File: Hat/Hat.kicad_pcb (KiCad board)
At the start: 2 copper layers, 185.8 x 128.5 mm, 102 parts, among them J1 Conn_01x01_Pin, J2 Conn_01x12_Pin, J3 Conn_01x12_Pin, J4 Conn_01x06_Pin, J5 Conn_01x01_Pin, Q1 BC547, Q10 BC547, Q11 BC547, Q12 BC557, Q13 BC547, Q14 BC547, Q15 BC547, Q2 BC547, Q3 BC547, Q4 BC557, Q5 BC557, Q6 BC547, Q7 BC547, Q8 BC547, Q9 BC547, SW1 SW_Push, SW2 SW_SPDT, U1 TL074, U2 Aux_flush, U3 Aux_flush, U4 Aux_flush, U5 4066, U6 Aux_flush, U7 Aux_flush

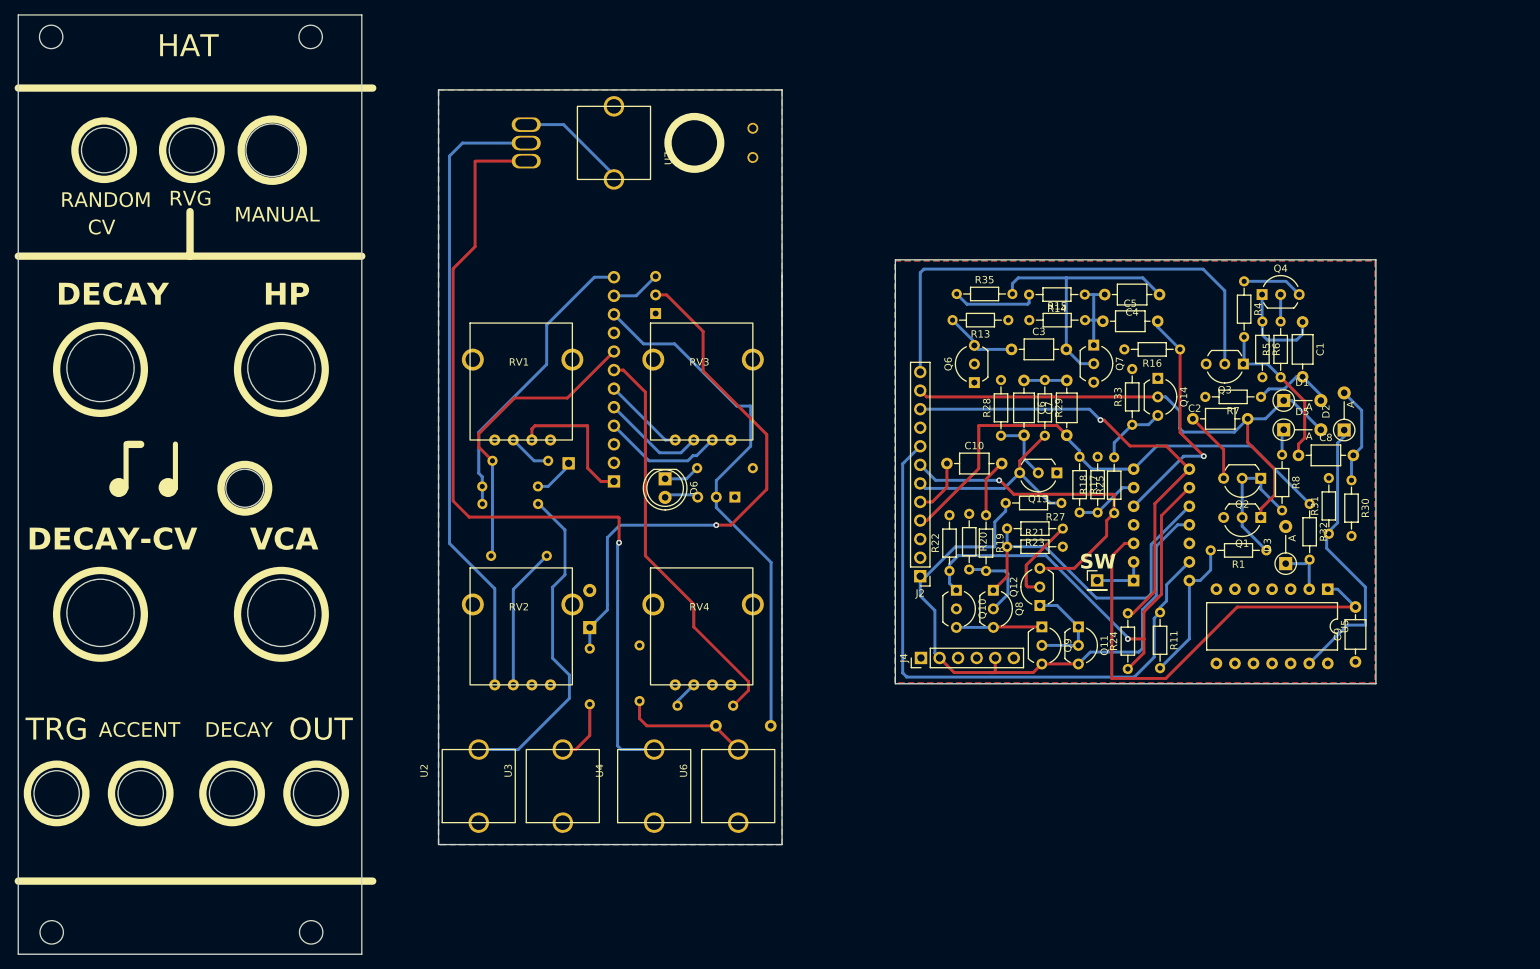
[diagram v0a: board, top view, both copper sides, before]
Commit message: Add files via upload
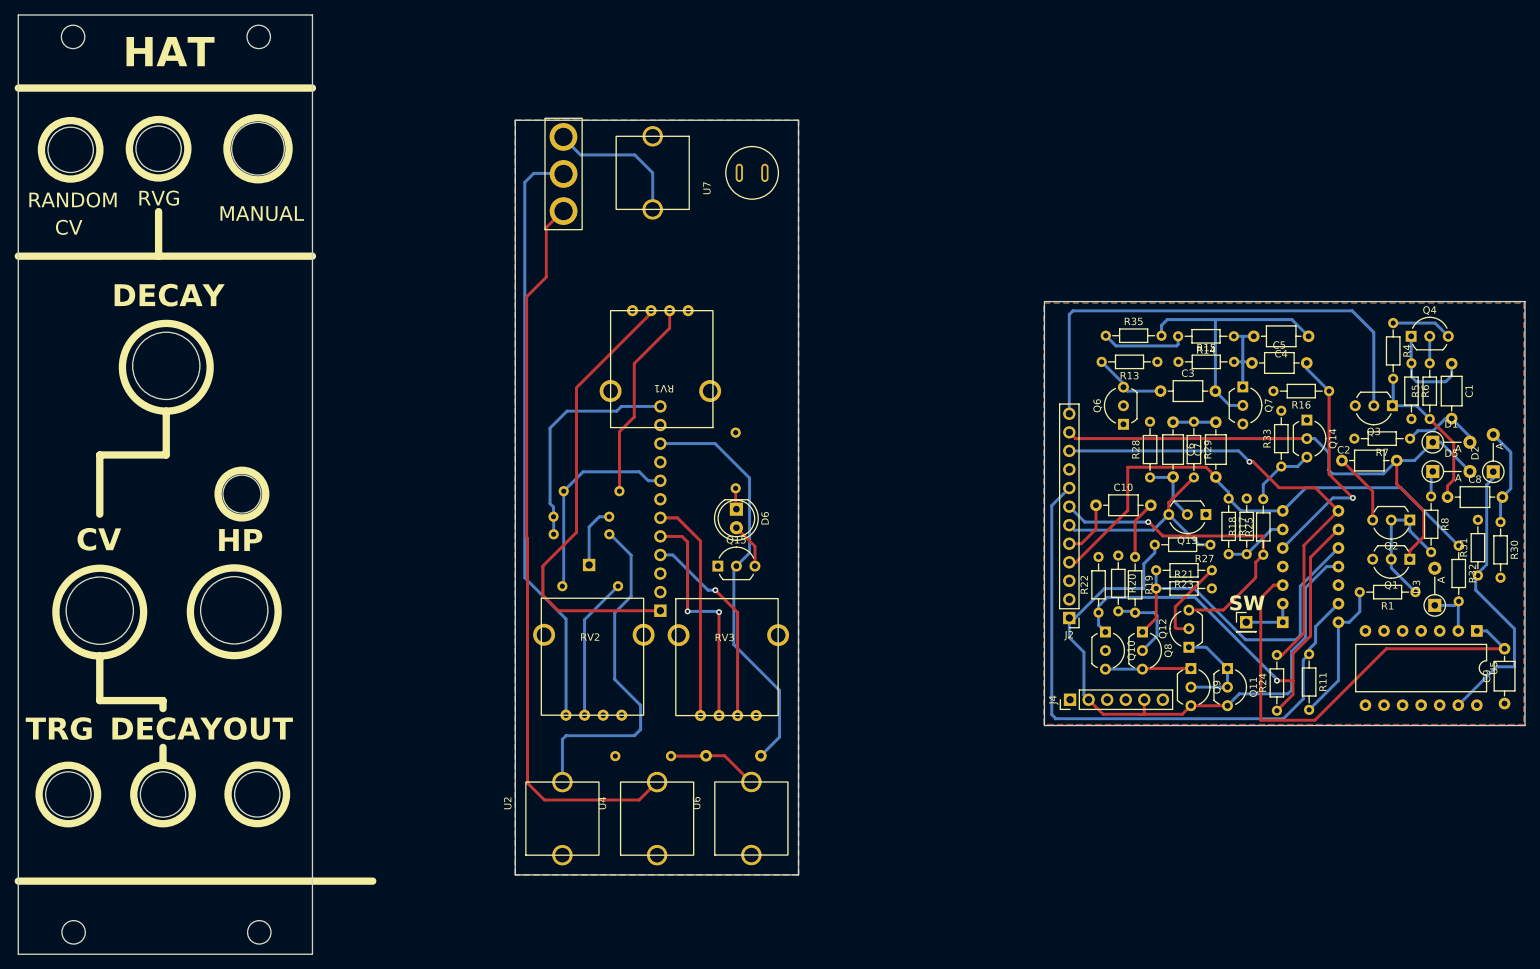
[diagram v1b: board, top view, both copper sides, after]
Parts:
- removed D4: D, Diode_THT:D_A-405_P5.08mm_Vertical_AnodeUp
- removed Q5: BC557, Package_TO_SOT_THT:TO-92_Inline_Wide
- removed R26: 100k, Resistor_THT:R_Axial_DIN0204_L3.6mm_D1.6mm_P7.62mm_Horizontal
- removed R9: 1k, Resistor_THT:R_Axial_DIN0204_L3.6mm_D1.6mm_P7.62mm_Horizontal
- removed the REF** at (59.2, 127.0)
- removed the REF** at (78.5, 68.8)
- removed RV4: R_Potentiometer, Library:AlpsPot
- removed U3: Aux_flush, Library:3mm5 Mono Aux
- Q15: moved to F.Cu
- SW1: footprint Library:Push_Flush -> Library:PushButton
- SW2: footprint Library:SPDT Mini -> Library:Switch
- moved RV3 37.9 mm to (135.8, 116.3)
- moved RV1 31.8 mm to (134.2, 61.0), turned to 180 degrees
- moved C5 21.2 mm to (211.3, 68.1)
- moved D2 21.2 mm to (244.3, 83.0)
- moved D3 21.2 mm to (236.3, 101.3)
- moved J4 21.2 mm to (186.4, 114.2)
- moved Q10 21.2 mm to (191.2, 104.9)
- moved Q11 21.2 mm to (207.9, 109.9)
- moved Q14 21.2 mm to (218.8, 75.9)
- moved Q8 21.2 mm to (196.3, 104.9)
- moved Q9 21.2 mm to (202.9, 109.9)
- moved R11 21.2 mm to (219.1, 108.0)
- moved R19 21.2 mm to (195.3, 94.7)
- moved R23 21.2 mm to (205.8, 96.5)
- moved R27 21.2 mm to (205.6, 93.0)
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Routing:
- net Net-(D4-K): track 74.5 -> 0.00 mm, vias 1 -> 0
- net OFFSET: track 100.4 -> 45.2 mm
- net -12V: track 103.3 -> 145.9 mm
- net Net-(R10-Pad1): track 5.95 -> 27.5 mm
- net NOISE_HP: track 40.0 -> 59.4 mm
- net NOISE_TONED: track 22.0 -> 39.8 mm, vias 0 -> 2
- net OUT: track 136.9 -> 120.6 mm
- net Net-(SW2-A): track 114.8 -> 100.9 mm, vias 1 -> 0
- net VGND: track 123.5 -> 110.7 mm
- net NOISE: track 86.5 -> 97.8 mm, vias 0 -> 1
- net IN: track 107.2 -> 97.8 mm
- net Net-(R9-Pad2): track 8.74 -> 0.00 mm
- net CAP: track 84.6 -> 77.8 mm
- net Net-(C11-Pad2): track 17.8 -> 12.5 mm
- net Net-(SW2-B): track 86.2 -> 81.1 mm
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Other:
- board size 185.8 x 128.5 mm -> 206.1 x 128.5 mm
- board text removed: "ACCENT"
- board text removed: "DECAY-CV"
- board text removed: "VCA"
